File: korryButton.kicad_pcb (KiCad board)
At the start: 2 copper layers, 30 x 30 mm, 14 parts, among them CN1 B5B-XH-A (LF)(SN), SW1 5.8 ZSGT, U1 SN74AHCT125DR, U3 WS2811C, U4 WS2811C

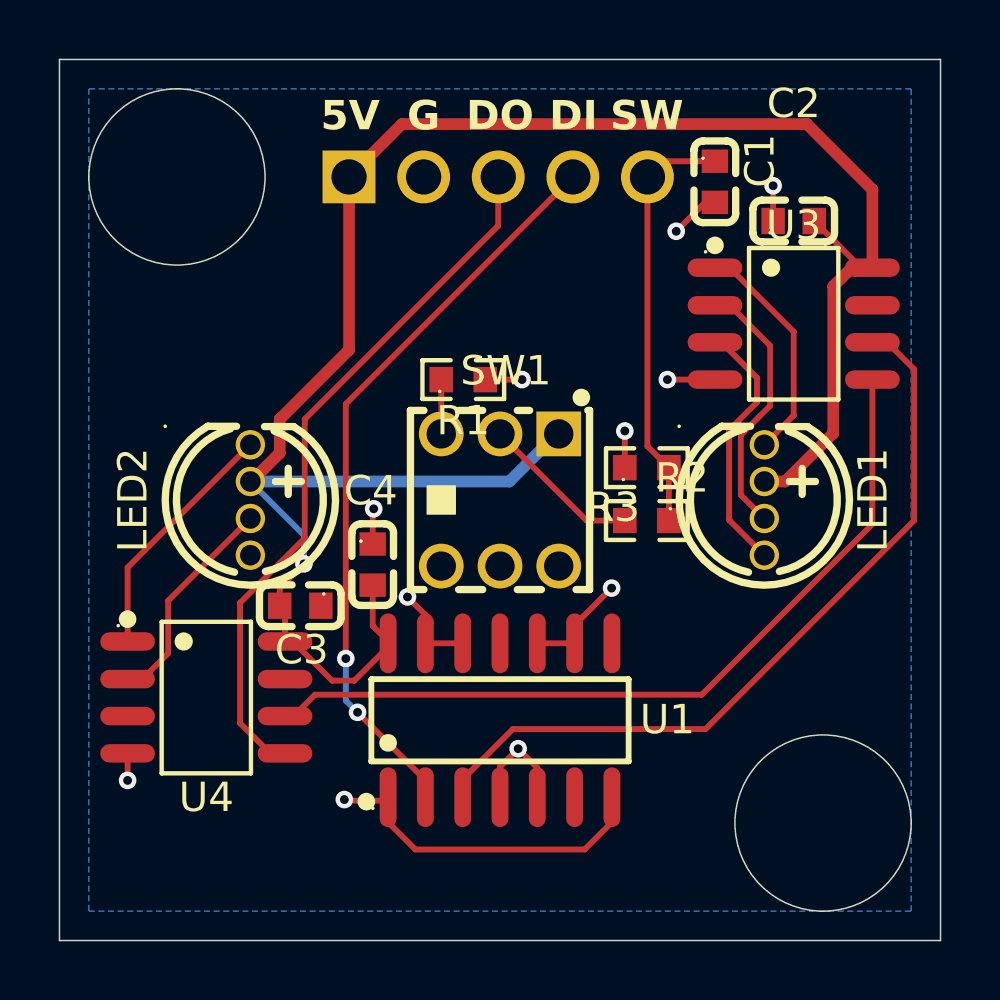
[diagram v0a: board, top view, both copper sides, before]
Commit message: update pcb for prod, prod finished
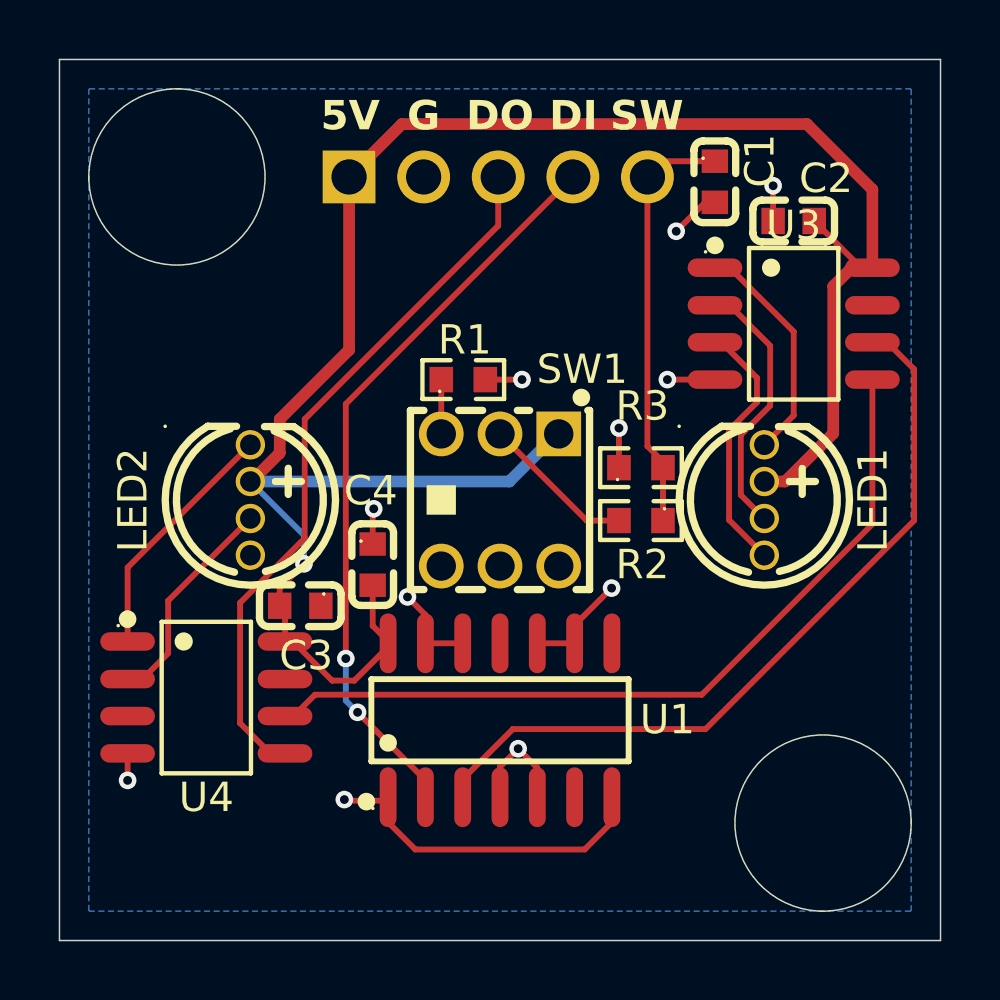
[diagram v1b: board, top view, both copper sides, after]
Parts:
- moved R2 0.20 mm to (104.8, 125.7)
- moved R3 0.20 mm to (104.8, 123.9)
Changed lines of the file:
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@@
 	(footprint "lcsc_footprints:C105575_R0603"
 		(layer "F.Cu")
-		(at 105 123.9)
+		(at 104.8 123.9)
 		(property "Reference" "R3"
-			(at -1.15 1.35 0)
+			(at 0.05 -2.1 0)
 			(layer "F.SilkS")
 			(effects
@@
 	(footprint "lcsc_footprints:C98220_R0603"
 		(layer "F.Cu")
-		(at 105 125.7 180)
+		(at 104.8 125.7 180)
 		(property "Reference" "R2"
-			(at -1.2 1.45 0)
+			(at -0.05 -1.5 0)
 			(layer "F.SilkS")
 			(effects
@@
 		(at 98.75 120.9)
 		(property "Reference" "R1"
-			(at 0 1.4 0)
+			(at 0.05 -1.35 0)
 			(layer "F.SilkS")
 			(effects
@@
 		(descr "100nF (104) ±10% 50V")
 		(property "Reference" "C3"
-			(at -0.05 -1.5 0)
+			(at -0.2 -1.7 0)
 			(layer "F.SilkS")
 			(effects
@@
 		(at 100 125)
 		(property "Reference" "SW1"
-			(at 0.2 -4.4 180)
+			(at 2.8 -4.45 180)
 			(layer "F.SilkS")
 			(effects
@@
 		(descr "100nF (104) ±10% 50V")
 		(property "Reference" "C2"
-			(at 0 -4 0)
+			(at 1.1 -1.45 0)
 			(layer "F.SilkS")
 			(effects
@@
 			)
 		)
-		(attr through_hole)
+		(attr through_hole exclude_from_pos_files exclude_from_bom dnp)
 		(duplicate_pad_numbers_are_jumpers no)
 		(fp_line
@@
 	)
 	(segment
-		(start 104.25 123.9)
-		(end 104.25 122.65)
-		(width 0.2)
-		(layer "F.Cu")
-		(net "GND")
-	)
-	(segment
 		(start 102.54 129.26)
 		(end 103.8 128)
@@
 	)
 	(segment
+		(start 104.05 123.9)
+		(end 104.05 122.55)
+		(width 0.2)
+		(layer "F.Cu")
+		(net "GND")
+	)
+	(segment
 		(start 102.54 129.88)
 		(end 102.54 129.26)
@@
 	)
 	(via
-		(at 104.25 122.65)
+		(at 87.32 134.5475)
 		(size 0.6)
 		(drill 0.3)
@@
 	)
 	(via
-		(at 87.32 134.5475)
+		(at 109.3 114.3)
 		(size 0.6)
 		(drill 0.3)
@@
 	)
 	(via
-		(at 109.3 114.3)
+		(at 104.05 122.55)
 		(size 0.6)
 		(drill 0.3)
@@
 	)
 	(segment
-		(start 105.75 125.7)
-		(end 105.75 123.9)
-		(width 0.2)
-		(layer "F.Cu")
-		(net "Net-(C1-Pad1)")
-	)
-	(segment
 		(start 107.315 113.465)
 		(end 105.555 113.465)
@@
 	(segment
 		(start 105.02 123.17)
-		(end 105.75 123.9)
+		(end 105.55 123.7)
+		(width 0.2)
+		(layer "F.Cu")
+		(net "Net-(C1-Pad1)")
+	)
+	(segment
+		(start 105.55 123.7)
+		(end 105.55 123.9)
 		(width 0.2)
 		(layer "F.Cu")
@@
 	)
 	(segment
+		(start 105.55 125.7)
+		(end 105.55 123.9)
+		(width 0.2)
+		(layer "F.Cu")
+		(net "Net-(C1-Pad1)")
+	)
+	(segment
 		(start 104.65 114.37)
 		(end 105.02 114)
@@
 	)
 	(segment
-		(start 102.95 125.7)
-		(end 104.25 125.7)
+		(start 100 122.75)
+		(end 102.95 125.7)
 		(width 0.2)
 		(layer "F.Cu")
@@
 	)
 	(segment
-		(start 100 122.75)
+		(start 104.05 125.7)
 		(end 102.95 125.7)
 		(width 0.2)
